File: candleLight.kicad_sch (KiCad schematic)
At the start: 44 parts, among them J1 USB_C_Receptacle_USB2.0, J2 Conn_Phoenix, J3 Conn_SWD, J4 Conn_3.3V, U1 ME6210A33PG, U2 STM32F072C8Tx, U3 TJA1051/3, Y1 8MHz

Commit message: LCSC
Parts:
- C1, C10, C2: LCSC (none) -> C440198; MPN C440198 -> (none)
- C11, C12, C5, C6, C7, C8, C9: LCSC (none) -> C14663; MPN C14663 -> (none)
- C3, C4: LCSC (none) -> C1658; MPN C1658 -> (none)
- D1, D2: LCSC (none) -> C2290; MPN C2290 -> (none)
- D3: LCSC (none) -> C2286; MPN C2286 -> (none)
- R1, R2: LCSC (none) -> C23162; MPN C23162 -> (none)
- R10, R4, R8, R9: LCSC (none) -> C21190; MPN C21190 -> (none)
- R11, R5: LCSC (none) -> C23186; MPN C23186 -> (none)
- R6: LCSC (none) -> C25804; MPN C25804 -> (none)
- U1: LCSC (none) -> C85233; MPN C85233 -> (none)
- U2: LCSC (none) -> C80488; MPN C80488 -> (none)
- U3: LCSC (none) -> C58988; MPN C58988 -> (none)
- Y1: LCSC (none) -> C144380; MPN C144380 -> (none)
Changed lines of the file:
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@@
 			)
 		)
-		(property "MPN" "C2290"
+		(property "LCSC" "C2290"
 			(at 262.89 30.48 0)
 			(effects
@@
 			)
 		)
-		(property "MPN" "C25804"
+		(property "LCSC" "C25804"
 			(at 157.48 35.56 90)
 			(effects
@@
 			)
 		)
-		(property "MPN" "C14663"
+		(property "LCSC" "C14663"
 			(at 55.88 27.94 0)
 			(effects
@@
 			)
 		)
-		(property "MPN" "C440198"
+		(property "LCSC" "C440198"
 			(at 191.77 97.79 0)
 			(effects
@@
 			)
 		)
-		(property "MPN" "C21190"
+		(property "LCSC" "C21190"
 			(at 251.46 30.48 90)
 			(effects
@@
 			)
 		)
-		(property "MPN" "C14663"
+		(property "LCSC" "C14663"
 			(at 48.26 27.94 0)
 			(effects
@@
 			)
 		)
-		(property "MPN" "C23162"
+		(property "LCSC" "C23162"
 			(at 53.34 90.17 90)
 			(effects
@@
 			)
 		)
-		(property "MPN" "C14663"
+		(property "LCSC" "C14663"
 			(at 163.83 57.15 0)
 			(effects
@@
 			)
 		)
-		(property "MPN" "C14663"
+		(property "LCSC" "C14663"
 			(at 156.21 57.15 0)
 			(effects
@@
 			)
 		)
-		(property "MPN" "C23186"
+		(property "LCSC" "C23186"
 			(at 55.88 157.48 90)
 			(effects
@@
 			)
 		)
-		(property "MPN" "C2286"
+		(property "LCSC" "C2286"
 			(at 262.89 48.26 0)
 			(effects
@@
 			)
 		)
-		(property "MPN" "C1658"
+		(property "LCSC" "C1658"
 			(at 63.5 54.61 90)
 			(effects
@@
 			)
 		)
-		(property "MPN" "C1658"
+		(property "LCSC" "C1658"
 			(at 63.5 59.69 90)
 			(effects
@@
 			)
 		)
-		(property "MPN" "C80488"
+		(property "LCSC" "C80488"
 			(at 104.14 77.47 0)
 			(effects
@@
 			)
 		)
-		(property "MPN" "C21190"
+		(property "LCSC" "C21190"
 			(at 46.99 54.61 90)
 			(effects
@@
 			)
 		)
-		(property "MPN" "C2290"
+		(property "LCSC" "C2290"
 			(at 262.89 39.37 0)
 			(effects
@@
 			)
 		)
-		(property "MPN" "C23186"
+		(property "LCSC" "C23186"
 			(at 55.88 152.4 90)
 			(effects
@@
 			)
 		)
-		(property "MPN" "C58988"
+		(property "LCSC" "C58988"
 			(at 190.5 35.56 0)
 			(effects
@@
 			)
 		)
-		(property "MPN" "C440198 "
+		(property "LCSC" "C440198 "
 			(at 74.93 27.94 0)
 			(effects
@@
 			)
 		)
-		(property "MPN" "C14663"
+		(property "LCSC" "C14663"
 			(at 63.5 27.94 0)
 			(effects
@@
 			)
 		)
-		(property "MPN" "C21190"
+		(property "LCSC" "C21190"
 			(at 251.46 39.37 90)
 			(effects
@@
 			)
 		)
-		(property "MPN" "C14663"
+		(property "LCSC" "C14663"
 			(at 40.64 27.94 0)
 			(effects
@@
 			)
 		)
-		(property "MPN" "C144380"
+		(property "LCSC" "C144380"
 			(at 69.85 57.15 0)
 			(effects
@@
 			)
 		)
-		(property "MPN" "C21190"
+		(property "LCSC" "C21190"
 			(at 251.46 48.26 90)
 			(effects
@@
 			)
 		)
-		(property "MPN" "C85233"
+		(property "LCSC" "C85233"
 			(at 179.07 92.71 0)
 			(effects
@@
 			)
 		)
-		(property "MPN" "C440198"
+		(property "LCSC" "C440198"
 			(at 163.83 92.71 0)
 			(effects
@@
 			)
 		)
-		(property "MPN" "C23162"
+		(property "LCSC" "C23162"
 			(at 53.34 87.63 90)
 			(effects
@@
 			)
 		)
-		(property "MPN" "C14663"
+		(property "LCSC" "C14663"
 			(at 29.21 48.26 0)
 			(effects

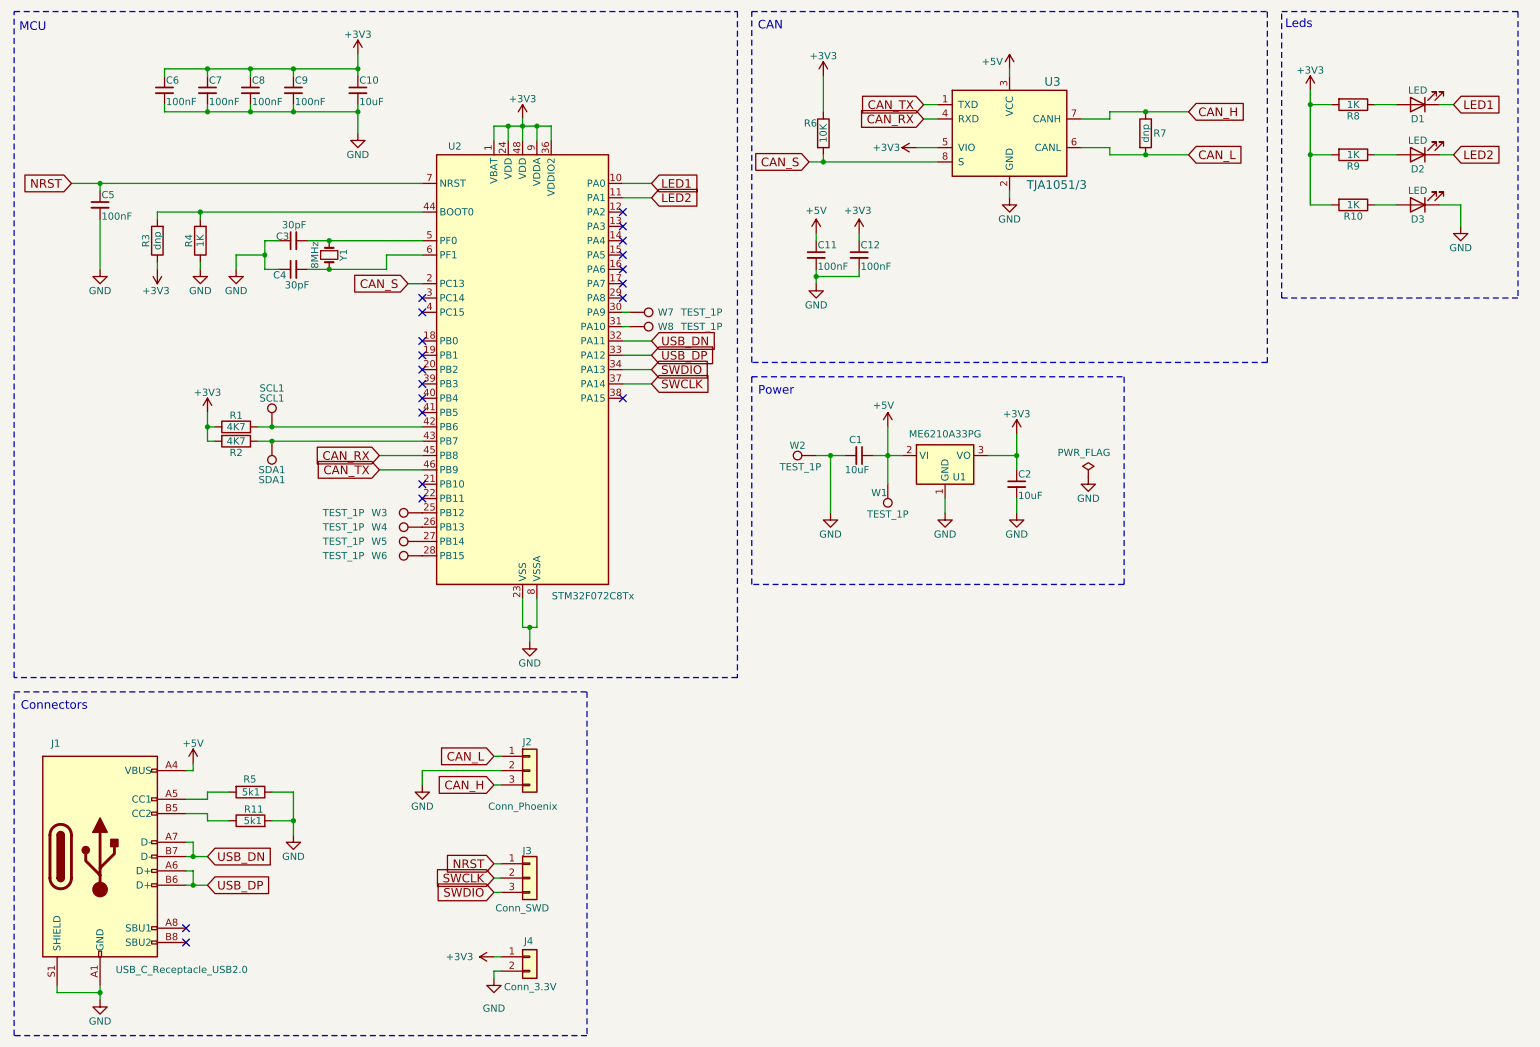
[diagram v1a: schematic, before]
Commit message: inital board
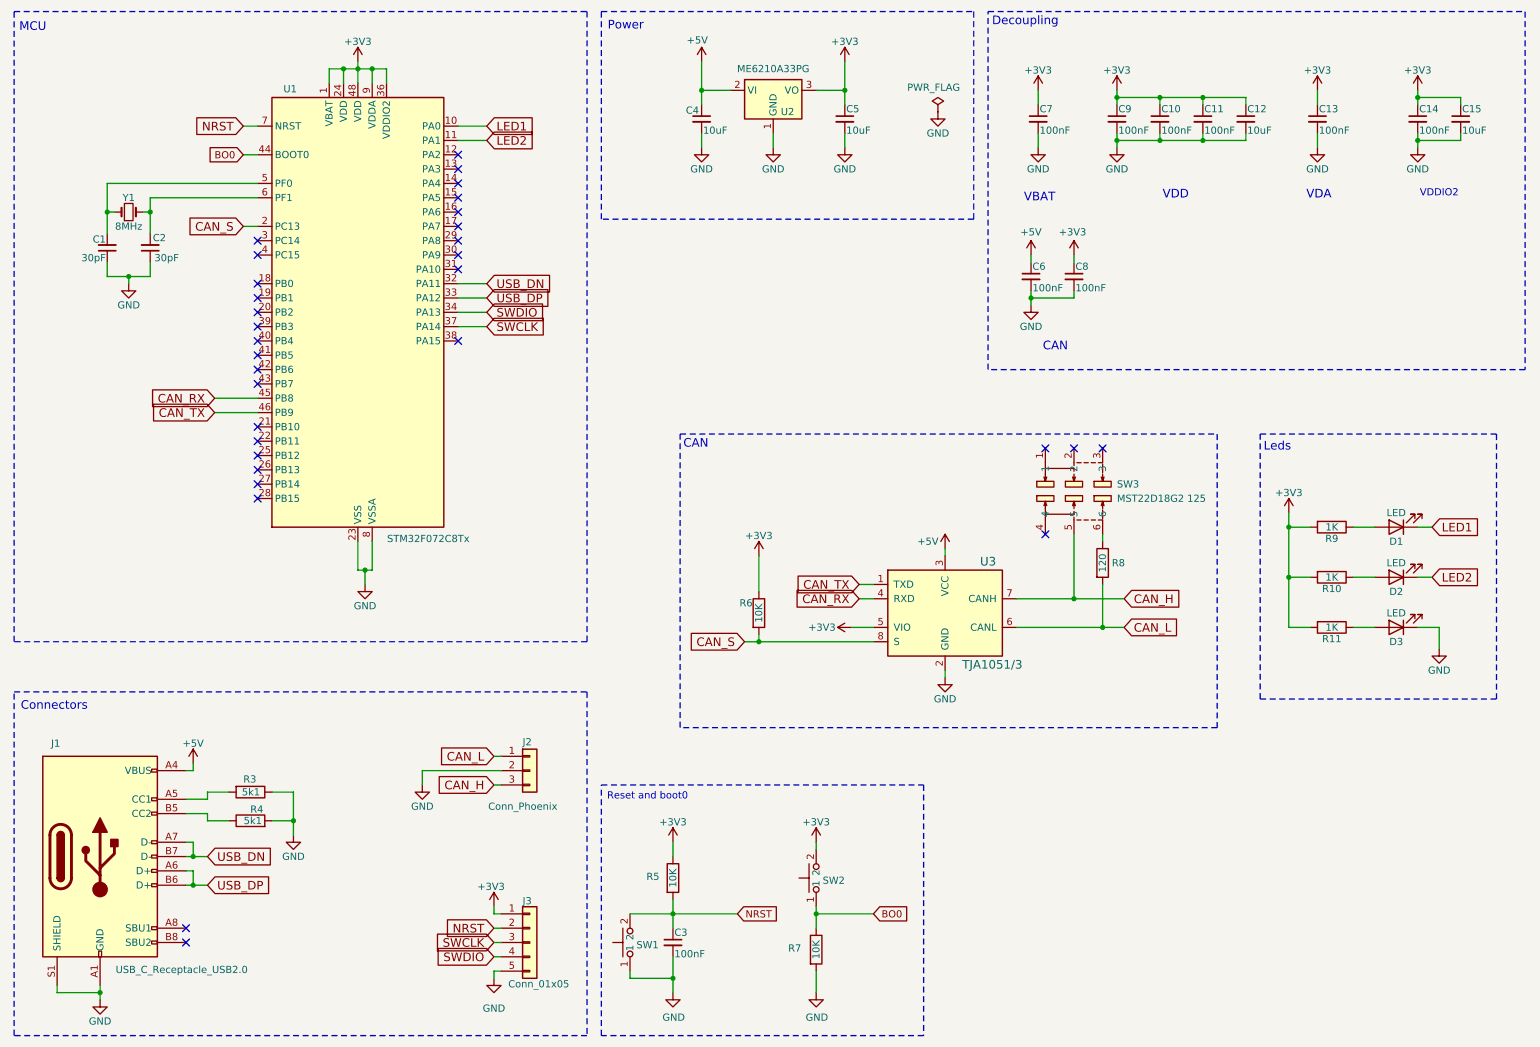
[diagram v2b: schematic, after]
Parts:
- removed C5: 100nF, Capacitor_SMD:C_0603_1608Metric, symbol Device:C_Small
- removed J3: Conn_SWD, Connector_PinHeader_2.54mm:PinHeader_1x03_P2.54mm_Vertical, symbol Connector_Generic:Conn_01x03
- removed J4: Conn_3.3V, Connector_PinHeader_2.54mm:PinHeader_1x02_P2.54mm_Vertical, symbol Connector_Generic:Conn_01x02
- removed R1, R2: 4K7, Resistor_SMD:R_0603_1608Metric, symbol Device:R
- removed R3: dnp, Resistor_SMD:R_0805_2012Metric, symbol Device:R
- removed R4: 1K, Resistor_SMD:R_0603_1608Metric, symbol Device:R
- removed SCL1: SCL1, Measurement_Points:Measurement_Point_Round-SMD-Pad_Small, symbol Connector:TestPoint
- removed SDA1: SDA1, Measurement_Points:Measurement_Point_Round-SMD-Pad_Small, symbol Connector:TestPoint
- removed W1, W2: TEST_1P, Measurement_Points:Measurement_Point_Round-SMD-Pad_Big, symbol Connector:TestPoint
- removed W3, W4, W5, W6, W7, W8: TEST_1P, Measurement_Points:Measurement_Point_Round-SMD-Pad_Small, symbol Connector:TestPoint
- added C13, C14, C3: 100nF, Capacitor_SMD:C_0603_1608Metric, symbol Device:C_Small
- added C15: 10uF, Capacitor_SMD:C_0805_2012Metric, symbol Device:C_Small
- added J3: Conn_01x05, Connector_PinHeader_2.54mm:PinHeader_1x05_P2.54mm_Vertical, symbol Connector_Generic:Conn_01x05
- added R5: 10K, Resistor_SMD:R_0603_1608Metric, symbol Device:R
- added R8: 120, Resistor_SMD:R_0603_1608Metric, symbol Device:R
- added SW1, SW2: TS-1088R-02526, stm32world:TS-1088R-02526, symbol stm32world:TS-1088R-02526
- added SW3: MST22D18G2 125, woldhack:SW-SMD_MST22D18G2, symbol woldhack:MST22D18G2125
- C1: renamed from C3; LCSC C1658 -> C1554
- C12: renamed from C10; LCSC C440198 -> C440198
- C2: renamed from C4; LCSC C1658 -> C1554
- R7: value dnp -> 10K; footprint Resistor_SMD:R_0805_2012Metric -> Resistor_SMD:R_0603_1608Metric; LCSC (none) -> C25804
- Y1: LCSC C144380 -> C115962
- renumbered C8 to C10, C9 to C11, C1 to C4, C2 to C5, C11 to C6, C6 to C7, C12 to C8, C7 to C9, R9 to R10, R10 to R11, R5 to R3, R11 to R4, R8 to R9, U2 to U1, U1 to U2
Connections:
- net +3V3: now also C13.1, C14.1, C15.1, J3.1 (Pin_1), R5.1, SW2.2
- net CAN_H: now also SW3.5; no longer R7.1
- net CAN_L: now also R8.2; no longer R7.2
- net GND: now also R7.2, C13.2, C14.2, C15.2, C3.2, J3.5 (Pin_5), SW1.1
- net NRST: now also C3.1, J3.2 (Pin_2), R5.2, SW1.2
- net SWCLK: now also J3.3 (Pin_3)
- net SWDIO: now also J3.4 (Pin_4)
- net BO0: now reaches U1.44 (BOOT0)
- net BO0: now also R7.1, SW2.1
- new net: R8.1, SW3.6
- no-connect marks 20 -> 32
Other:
- note added: "Decoupling"
- note added: "Reset and boot0"
- note added: "VBAT"
- note added: "VDA"
- note added: "VDD"
- note added: "VDDIO2"
- moved on the sheet: C1, C10, C11, C12, C2, C4, C5, C6, C7, C8, C9, D1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

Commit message: layout
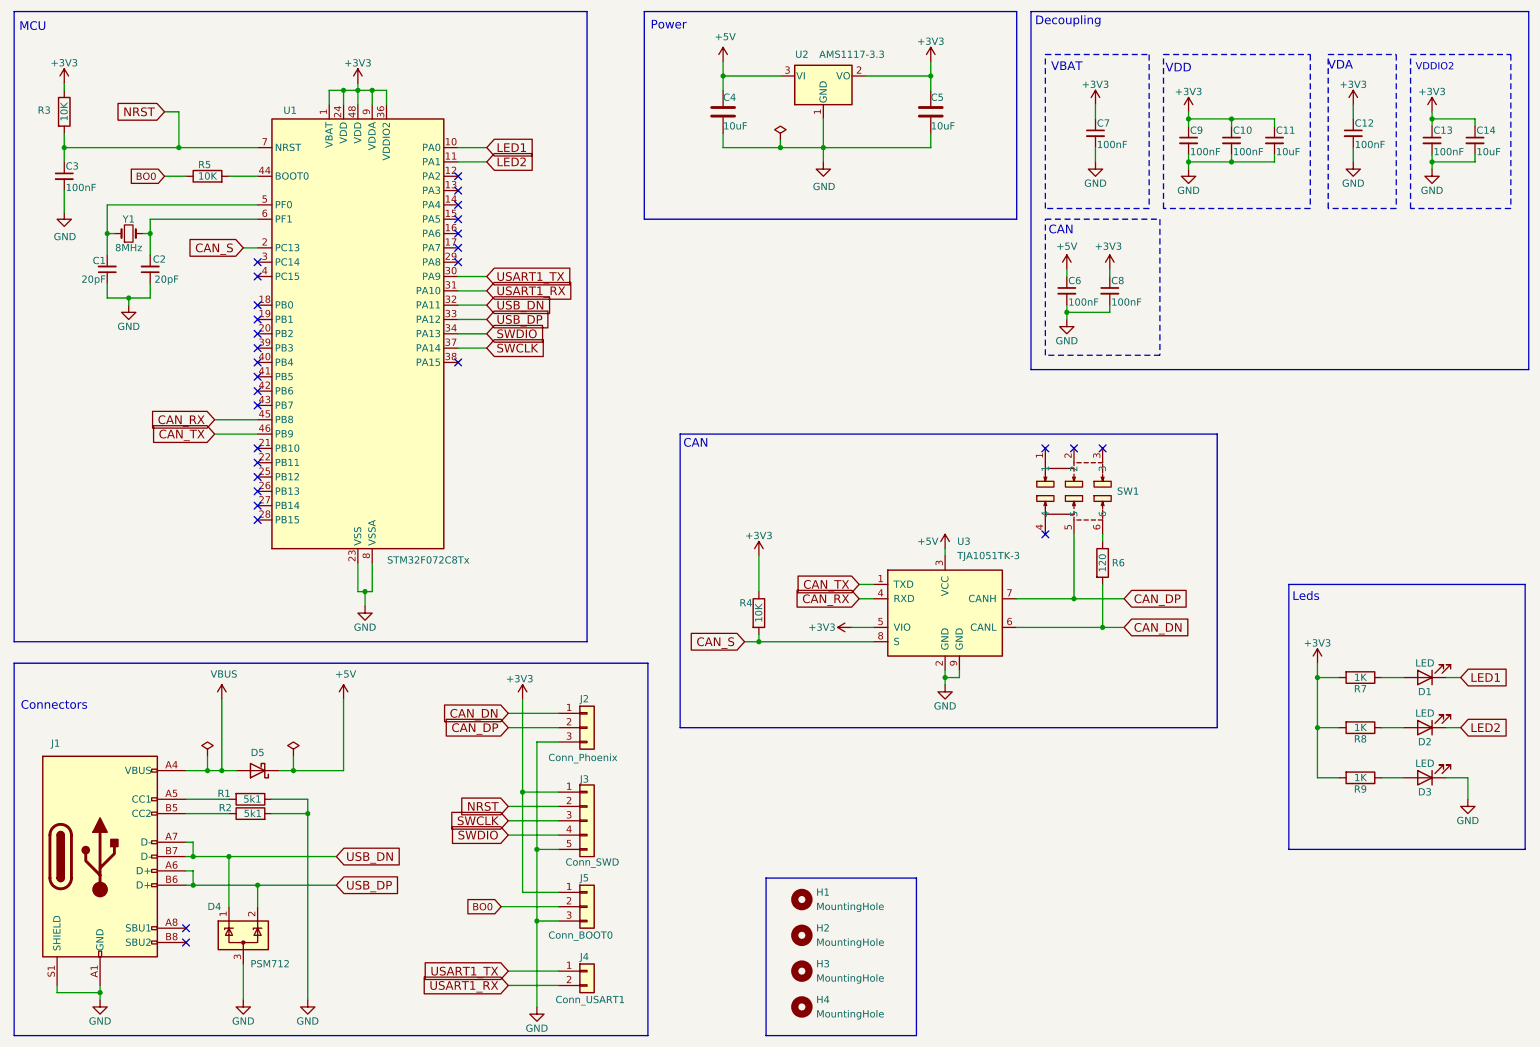
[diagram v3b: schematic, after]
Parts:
- removed C11: 100nF, Capacitor_SMD:C_0603_1608Metric, symbol Device:C_Small
- removed C4, C5: 10uF, Capacitor_SMD:C_0805_2012Metric, symbol Device:C_Small
- removed SW1, SW2: TS-1088R-02526, stm32world:TS-1088R-02526, symbol stm32world:TS-1088R-02526
- removed U2: ME6210A33PG, Package_TO_SOT_SMD:SOT-89-3, symbol Regulator_Linear:MCP1754S-1802xMB
- removed U3: TJA1051/3, Package_SO:SOIC-8_3.9x4.9mm_P1.27mm, symbol Interface_CAN_LIN:TJA1051T-3
- added C4, C5: C_10UF_0805, Capacitor_SMD:C_0805_2012Metric, symbol stm32world:C_10UF_0805
- added D4: PSM712, Package_TO_SOT_SMD:SOT-23, symbol Power_Protection:SP0502BAHT
- added D5: ~, Diode_SMD:D_SOD-123, symbol Device:D_Schottky
- added H1, H2, H3, H4: MountingHole, MountingHole:MountingHole_2.1mm, symbol Mechanical:MountingHole
- added J4: Conn_USART1, Connector_PinHeader_2.54mm:PinHeader_1x02_P2.54mm_Vertical, symbol Connector_Generic:Conn_01x02
- added J5: Conn_BOOT0, Connector_PinHeader_2.54mm:PinHeader_1x03_P2.54mm_Vertical, symbol Connector_Generic:Conn_01x03
- added U2: AMS1117-3.3, Package_TO_SOT_SMD:SOT-223-3_TabPin2, symbol stm32world:AMS1117-3.3
- added U3: TJA1051TK-3, Package_DFN_QFN:DFN-8-1EP_3x3mm_P0.65mm_EP1.55x2.4mm, symbol Interface_CAN_LIN:TJA1051TK-3
- C1, C2: value 30pF -> 20pF
- J3: value Conn_01x05 -> Conn_SWD
- renumbered C12 to C11, C13 to C12, C14 to C13, C15 to C14, R3 to R1, R4 to R2, R5 to R3, R6 to R4, R7 to R5, R8 to R6, R9 to R7, R10 to R8, R11 to R9, SW3 to SW1
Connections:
- net +3V3: now also C5.1, J5.1 (Pin_1), U2.2 (VO), U3.5 (VIO)
- net +5V: now also C4.1, D5.1 (K), U2.3 (VI), U3.3 (VCC); no longer J1.A4 (VBUS), J1.A9 (VBUS), J1.B4 (VBUS), J1.B9 (VBUS)
- net BO0: now also J5.2 (Pin_2); no longer U1.44 (BOOT0)
- net CAN_RX: now also U3.4 (RXD)
- net CAN_S: now also U3.8 (S)
- net CAN_TX: now also U3.1 (TXD)
- net GND: now also J2.3 (Pin_3), C4.2, C5.2, D4.3 (A), J5.3 (Pin_3), U2.1 (GND), U3.2 (GND), U3.9 (GND); no longer J2.2 (Pin_2), R5.2
- net USB_DN: now also D4.1 (K)
- net USB_DP: now also D4.2 (K)
- net USART1_TX: now reaches U1.30 (PA9)
- net USART1_TX: now also J4.1 (Pin_1)
- net USART1_RX: now reaches U1.31 (PA10)
- net USART1_RX: now also J4.2 (Pin_2)
- net CAN_H renamed CAN_DP
- net CAN_DP: now also J2.2 (Pin_2), U3.7 (CANH); no longer J2.3 (Pin_3)
- net CAN_L renamed CAN_DN
- net CAN_DN: now also U3.6 (CANL)
- new net: R5.2, U1.44 (BOOT0)
- new net VBUS: D5.2 (A), J1.A4 (VBUS), J1.A9 (VBUS), J1.B4 (VBUS), J1.B9 (VBUS)
- no-connect marks 32 -> 30
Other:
- note removed: "Reset and boot0"
- moved on the sheet: C1, C10, C11, C12, C13, C14, C2, C3, C6, C7, C8, C9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
